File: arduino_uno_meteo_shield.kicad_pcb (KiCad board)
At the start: 2 copper layers, 14 parts

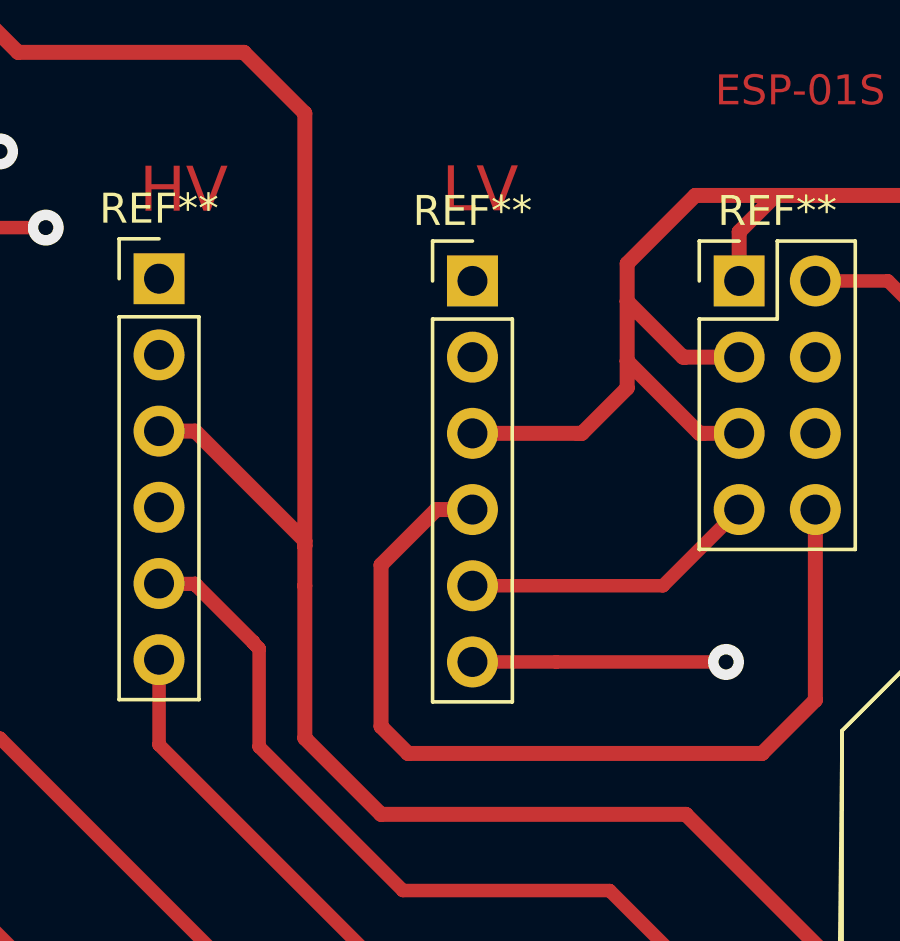
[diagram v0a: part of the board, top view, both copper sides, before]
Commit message: logic gate fix roaster
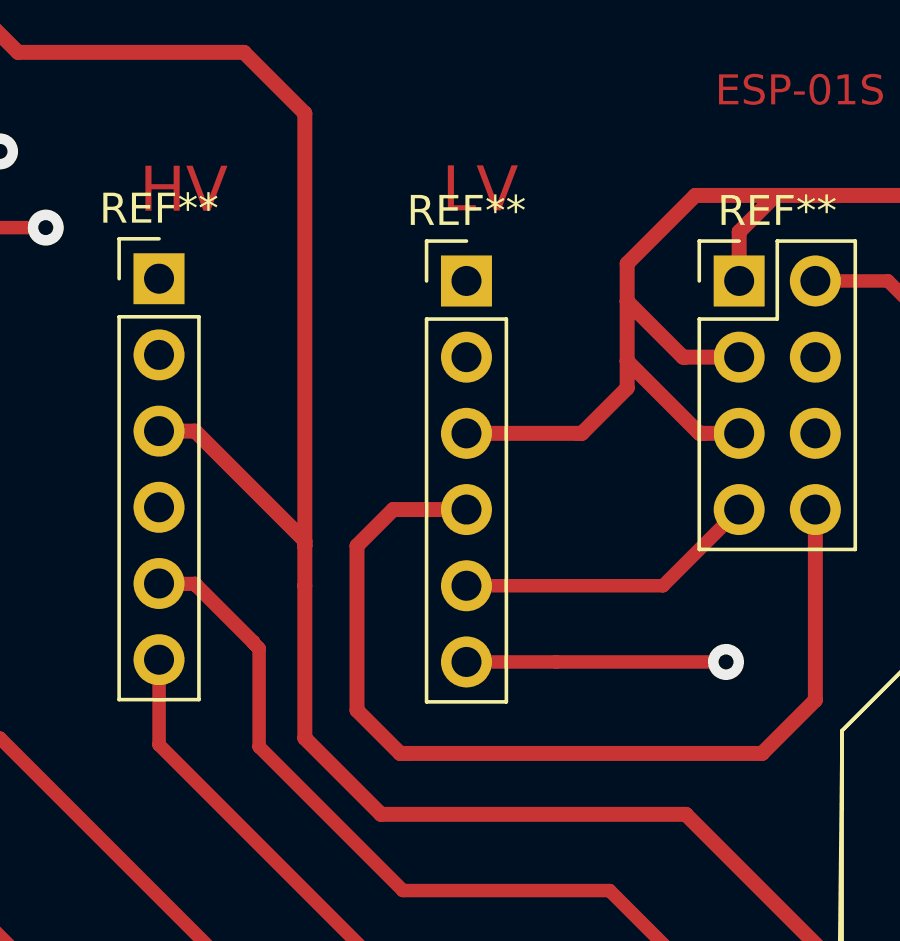
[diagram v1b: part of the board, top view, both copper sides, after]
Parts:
- moved REF** 0.20 mm to (167.9, 88.9)
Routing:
- net (no net): track 938.4 -> 939.9 mm
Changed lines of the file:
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@@
     (thickness 1.6)
     (drawings 21)
-    (tracks 251)
+    (tracks 252)
     (zones 0)
     (modules 14)
@@
   )
   (setup
-    (last_trace_width 0.45)
+    (last_trace_width 0.5)
     (user_trace_width 0.25)
     (user_trace_width 0.35)
@@
     (mod_text_width 0.15)
     (pad_size 1.7 1.7)
-    (pad_drill 1)
+    (pad_drill 0)
     (pad_to_mask_clearance 0.051)
     (solder_mask_min_width 0.25)
@@
     (pad 1 thru_hole rect (at 0 0) (size 1.7 1.7) (drill 1) (layers *.Cu *.Mask))
     (pad 2 thru_hole oval (at 0 2.54) (size 1.7 1.7) (drill 1) (layers *.Cu *.Mask))
-    (pad 3 thru_hole oval (at 0 5.08) (size 1.7 1.7) (drill 1) (layers *.Cu *.Mask))
+    (pad GND thru_hole oval (at 0 5.08) (size 1.7 1.7) (drill 1) (layers *.Cu *.Mask))
     (model ${KISYS3DMOD}/Connector_PinHeader_2.54mm.3dshapes/PinHeader_1x03_P2.54mm_Vertical.wrl
       (at (xyz 0 0 0))
@@
       (effects (font (size 1 1) (thickness 0.15)))
     )
-    (pad 1 thru_hole circle (at 0 0) (size 1.7 1.7) (drill 1) (layers *.Cu *.Mask))
+    (pad GND thru_hole circle (at 0 0) (size 1.7 1.7) (drill 1) (layers *.Cu *.Mask))
     (model ${KISYS3DMOD}/Connector_PinHeader_2.54mm.3dshapes/PinHeader_1x01_P2.54mm_Vertical.wrl
       (at (xyz 0 0 0))
@@
     (fp_line (start 1.27 -1.27) (end 1.27 39.37) (layer F.Fab) (width 0.1))
     (fp_line (start -0.635 -1.27) (end 1.27 -1.27) (layer F.Fab) (width 0.1))
-    (pad 16 thru_hole oval (at 0 38.1 90) (size 1.7 1.7) (drill 1) (layers *.Cu *.Mask))
+    (pad GND thru_hole oval (at 0 38.1 90) (size 1.7 1.7) (drill 1) (layers *.Cu *.Mask))
     (pad 15 thru_hole oval (at 0 35.56 90) (size 1.7 1.7) (drill 1) (layers *.Cu *.Mask))
     (pad 14 thru_hole oval (at 0 33.02 90) (size 1.7 1.7) (drill 1) (layers *.Cu *.Mask))
@@
     (pad 7 thru_hole oval (at 0 15.24 90) (size 1.7 1.7) (drill 1) (layers *.Cu *.Mask))
     (pad 6 thru_hole oval (at 0 12.7 90) (size 1.7 1.7) (drill 1) (layers *.Cu *.Mask))
-    (pad 5 thru_hole oval (at 0 10.16 90) (size 1.7 1.7) (drill 1) (layers *.Cu *.Mask))
+    (pad GND thru_hole oval (at 0 10.16 90) (size 1.7 1.7) (drill 1) (layers *.Cu *.Mask))
     (pad 4 thru_hole oval (at 0 7.62 90) (size 1.7 1.7) (drill 1) (layers *.Cu *.Mask))
     (pad 3 thru_hole oval (at 0 5.08 90) (size 1.7 1.7) (drill 1) (layers *.Cu *.Mask))
     (pad 2 thru_hole oval (at 0 2.54 90) (size 1.7 1.7) (drill 1) (layers *.Cu *.Mask))
-    (pad 1 thru_hole rect (at 0 0 90) (size 1.7 1.7) (drill 1) (layers *.Cu *.Mask))
+    (pad GND thru_hole rect (at 0 0 90) (size 1.7 1.7) (drill 1) (layers *.Cu *.Mask))
     (model ${KISYS3DMOD}/Connector_PinHeader_2.54mm.3dshapes/PinHeader_1x16_P2.54mm_Vertical.wrl
       (at (xyz 0 0 0))
@@
     (pad 6 thru_hole oval (at 0 12.7) (size 1.7 1.7) (drill 1) (layers *.Cu *.Mask))
     (pad 5 thru_hole oval (at 0 10.16) (size 1.7 1.7) (drill 1) (layers *.Cu *.Mask))
-    (pad 4 thru_hole oval (at 0 7.62) (size 1.7 1.7) (drill 1) (layers *.Cu *.Mask))
+    (pad GND thru_hole oval (at 0 7.62) (size 1.7 1.7) (drill 1) (layers *.Cu *.Mask))
     (pad 3 thru_hole oval (at 0 5.08) (size 1.7 1.7) (drill 1) (layers *.Cu *.Mask))
     (pad 2 thru_hole oval (at 0 2.54) (size 1.7 1.7) (drill 1) (layers *.Cu *.Mask))
@@
   )
   (module Connector_PinHeader_2.54mm:PinHeader_1x06_P2.54mm_Vertical (layer F.Cu)
-    (at 168.148 88.9)
+    (at 167.948 88.9)
     (descr "Through hole straight pin header, 1x06, 2.54mm pitch, single row")
     (tags "Through hole pin header THT 1x06 2.54mm single row")
@@
     (pad 3 thru_hole oval (at 0 5.08) (size 1.7 1.7) (drill 1) (layers *.Cu *.Mask))
     (pad 2 thru_hole oval (at 0 2.54) (size 1.7 1.7) (drill 1) (layers *.Cu *.Mask))
-    (pad 1 thru_hole rect (at 0 0) (size 1.7 1.7) (drill 1) (layers *.Cu *.Mask))
+    (pad GND thru_hole rect (at 0 0) (size 1.7 1.7) (drill 1) (layers *.Cu *.Mask))
     (model ${KISYS3DMOD}/Connector_PinHeader_2.54mm.3dshapes/PinHeader_1x03_P2.54mm_Vertical.wrl
       (at (xyz 0 0 0))
@@
     (pad 5 thru_hole oval (at 0 10.16) (size 1.7 1.7) (drill 1) (layers *.Cu *.Mask))
     (pad 4 thru_hole oval (at 0 7.62) (size 1.7 1.7) (drill 1) (layers *.Cu *.Mask))
-    (pad 3 thru_hole oval (at 0 5.08) (size 1.7 1.7) (drill 1) (layers *.Cu *.Mask))
+    (pad GND thru_hole oval (at 0 5.08) (size 1.7 1.7) (drill 1) (layers *.Cu *.Mask))
     (pad 2 thru_hole oval (at 0 2.54) (size 1.7 1.7) (drill 1) (layers *.Cu *.Mask))
     (pad 1 thru_hole rect (at 0 0) (size 1.7 1.7) (drill 1) (layers *.Cu *.Mask))
@@
     (pad 4 thru_hole oval (at 0 7.62) (size 1.7 1.7) (drill 1) (layers *.Cu *.Mask))
     (pad 3 thru_hole oval (at 0 5.08) (size 1.7 1.7) (drill 1) (layers *.Cu *.Mask))
-    (pad 2 thru_hole oval (at 0 2.54) (size 1.7 1.7) (drill 1) (layers *.Cu *.Mask))
+    (pad GND thru_hole oval (at 0 2.54) (size 1.7 1.7) (drill 1) (layers *.Cu *.Mask))
     (pad 1 thru_hole rect (at 0 0) (size 1.7 1.7) (drill 1) (layers *.Cu *.Mask))
     (model ${KISYS3DMOD}/Connector_PinHeader_2.54mm.3dshapes/PinHeader_1x04_P2.54mm_Vertical.wrl
@@
     (pad 4 thru_hole oval (at 0 7.62) (size 1.7 1.7) (drill 1) (layers *.Cu *.Mask))
     (pad 3 thru_hole oval (at 0 5.08) (size 1.7 1.7) (drill 1) (layers *.Cu *.Mask))
-    (pad 2 thru_hole oval (at 0 2.54) (size 1.7 1.7) (drill 1) (layers *.Cu *.Mask))
+    (pad GND thru_hole oval (at 0 2.54) (size 1.7 1.7) (drill 1) (layers *.Cu *.Mask))
     (pad 1 thru_hole rect (at 0 0) (size 1.7 1.7) (drill 1) (layers *.Cu *.Mask))
     (model ${KISYS3DMOD}/Connector_PinHeader_2.54mm.3dshapes/PinHeader_1x04_P2.54mm_Vertical.wrl
@@
   (segment (start 173.3042 91.5708) (end 173.3042 92.4708) (width 0.5) (layer F.Cu) (net 0))
   (segment (start 179.578 102.872) (end 179.578 96.52) (width 0.5) (layer F.Cu) (net 0))
-  (segment (start 166.945919 96.52) (end 165.1 98.365919) (width 0.5) (layer F.Cu) (net 0))
-  (segment (start 168.148 96.52) (end 166.945919 96.52) (width 0.5) (layer F.Cu) (net 0))
-  (segment (start 165.1 98.365919) (end 165.1 103.75) (width 0.5) (layer F.Cu) (net 0))
-  (segment (start 165.1 103.75) (end 166 104.65) (width 0.5) (layer F.Cu) (net 0))
   (segment (start 166 104.65) (end 177.8 104.65) (width 0.5) (layer F.Cu) (net 0))
   (segment (start 177.8 104.65) (end 179.578 102.872) (width 0.5) (layer F.Cu) (net 0))
@@
   (segment (start 132.588 101.6) (end 132.588 102.108) (width 0.45) (layer F.Cu) (net 0))
   (segment (start 132.588 101.6) (end 128.27 97.282) (width 0.45) (layer F.Cu) (net 0))
+  (segment (start 165.5064 96.52) (end 167.948 96.52) (width 0.5) (layer F.Cu) (net 0))
+  (segment (start 164.2999 97.7265) (end 165.5064 96.52) (width 0.5) (layer F.Cu) (net 0))
+  (segment (start 164.2999 103.2129) (end 164.2999 97.7265) (width 0.5) (layer F.Cu) (net 0))
+  (segment (start 166 104.65) (end 165.737 104.65) (width 0.5) (layer F.Cu) (net 0))
+  (segment (start 165.737 104.65) (end 164.2999 103.2129) (width 0.5) (layer F.Cu) (net 0))
   (zone (net 0) (net_name "") (layer F.Cu) (hatch edge 0.508)
     (connect_pads (clearance 0.508))

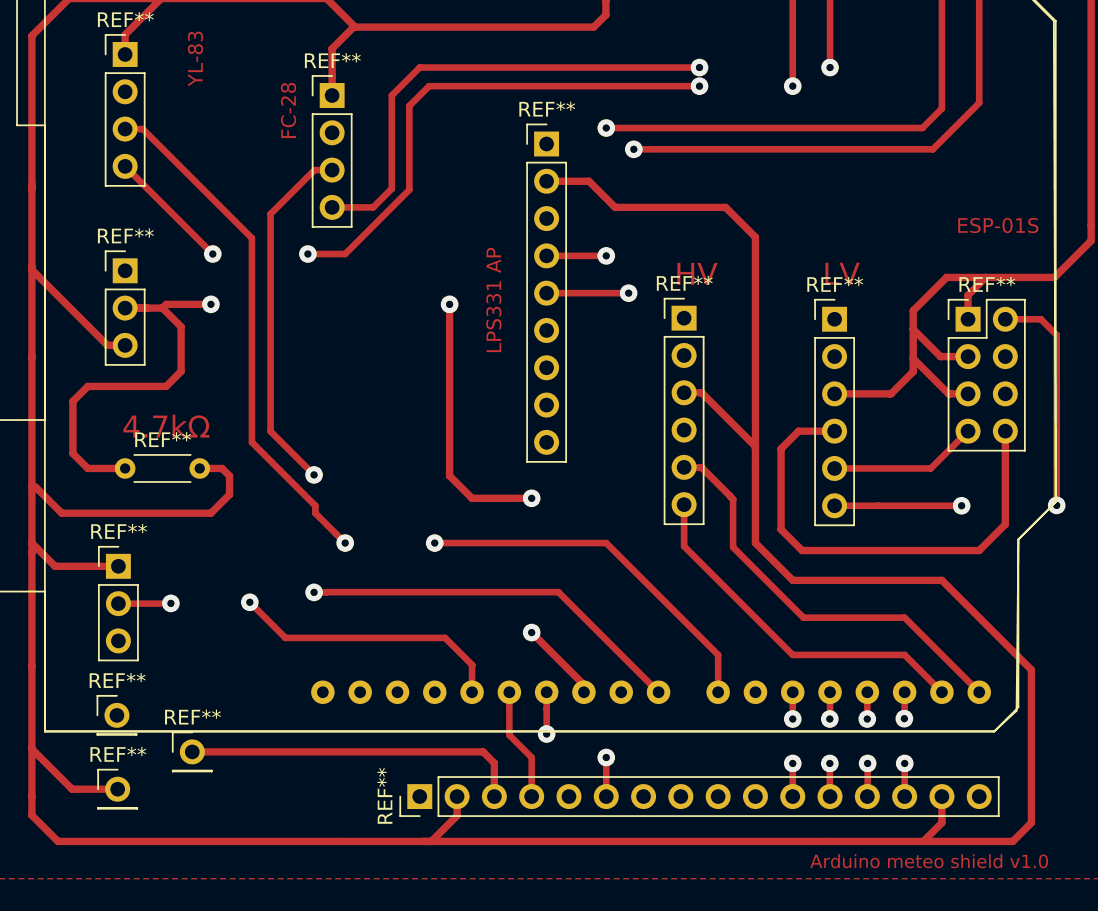
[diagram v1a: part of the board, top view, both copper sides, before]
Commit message: GND fix
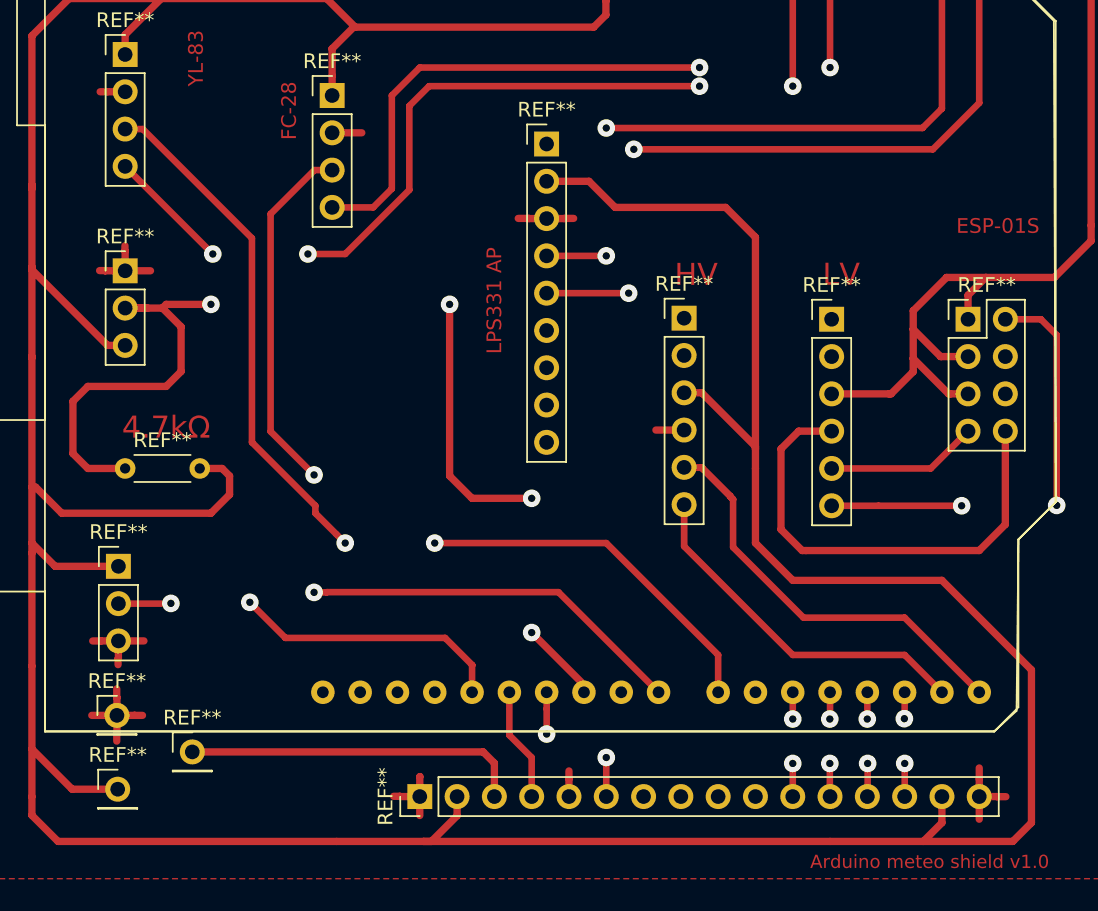
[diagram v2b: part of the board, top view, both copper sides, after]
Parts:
- moved REF** 0.20 mm to (167.7, 88.9)
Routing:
- net (no net): track 939.9 -> 978.1 mm
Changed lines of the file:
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@@
     (thickness 1.6)
     (drawings 21)
-    (tracks 252)
+    (tracks 300)
     (zones 0)
     (modules 14)
@@
   )
   (module Connector_PinHeader_2.54mm:PinHeader_1x06_P2.54mm_Vertical (layer F.Cu)
-    (at 167.948 88.9)
+    (at 167.748 88.9)
     (descr "Through hole straight pin header, 1x06, 2.54mm pitch, single row")
     (tags "Through hole pin header THT 1x06 2.54mm single row")
@@
   (segment (start 166 104.65) (end 165.737 104.65) (width 0.5) (layer F.Cu) (net 0))
   (segment (start 165.737 104.65) (end 164.2999 103.2129) (width 0.5) (layer F.Cu) (net 0))
+  (segment (start 119.634 73.406) (end 118.431919 73.406) (width 0.5) (layer F.Cu) (net 0))
+  (segment (start 118.431919 73.406) (end 117.9322 73.406) (width 0.5) (layer F.Cu) (net 0))
+  (segment (start 118.284 85.598) (end 118.2713 85.5853) (width 0.5) (layer F.Cu) (net 0))
+  (segment (start 119.634 85.598) (end 118.284 85.598) (width 0.5) (layer F.Cu) (net 0))
+  (segment (start 118.2713 85.5853) (end 117.8941 85.5853) (width 0.5) (layer F.Cu) (net 0))
+  (segment (start 119.634 85.598) (end 121.3612 85.598) (width 0.5) (layer F.Cu) (net 0))
+  (segment (start 119.634 84.248) (end 119.6213 84.2353) (width 0.5) (layer F.Cu) (net 0))
+  (segment (start 119.634 85.598) (end 119.634 84.248) (width 0.5) (layer F.Cu) (net 0))
+  (segment (start 119.6213 84.2353) (end 119.6213 83.8962) (width 0.5) (layer F.Cu) (net 0))
+  (segment (start 117.972919 110.805) (end 117.970419 110.8075) (width 0.5) (layer F.Cu) (net 0))
+  (segment (start 119.175 110.805) (end 117.972919 110.805) (width 0.5) (layer F.Cu) (net 0))
+  (segment (start 117.970419 110.8075) (end 117.4242 110.8075) (width 0.5) (layer F.Cu) (net 0))
+  (segment (start 119.175 110.805) (end 120.9142 110.805) (width 0.5) (layer F.Cu) (net 0))
+  (segment (start 119.175 112.007081) (end 119.1514 112.030681) (width 0.5) (layer F.Cu) (net 0))
+  (segment (start 119.175 110.805) (end 119.175 112.007081) (width 0.5) (layer F.Cu) (net 0))
+  (segment (start 119.1514 112.030681) (end 119.1514 112.4204) (width 0.5) (layer F.Cu) (net 0))
+  (segment (start 119.075 114.672919) (end 119.0625 114.660419) (width 0.5) (layer F.Cu) (net 0))
+  (segment (start 119.075 115.875) (end 119.075 114.672919) (width 0.5) (layer F.Cu) (net 0))
+  (segment (start 119.0625 114.660419) (end 119.0625 114.0714) (width 0.5) (layer F.Cu) (net 0))
+  (segment (start 119.075 117.077081) (end 119.0625 117.089581) (width 0.5) (layer F.Cu) (net 0))
+  (segment (start 119.075 115.875) (end 119.075 117.077081) (width 0.5) (layer F.Cu) (net 0))
+  (segment (start 119.0625 117.089581) (end 119.0625 117.6274) (width 0.5) (layer F.Cu) (net 0))
+  (segment (start 119.075 115.875) (end 117.3609 115.875) (width 0.5) (layer F.Cu) (net 0))
+  (segment (start 120.277081 115.875) (end 120.277281 115.8748) (width 0.5) (layer F.Cu) (net 0))
+  (segment (start 119.075 115.875) (end 120.277081 115.875) (width 0.5) (layer F.Cu) (net 0))
+  (segment (start 120.277281 115.8748) (end 120.8151 115.8748) (width 0.5) (layer F.Cu) (net 0))
+  (segment (start 138.35 121.404) (end 138.3326 121.3866) (width 0.5) (layer F.Cu) (net 0))
+  (segment (start 139.7 121.404) (end 138.35 121.404) (width 0.5) (layer F.Cu) (net 0))
+  (segment (start 138.3326 121.3866) (end 137.922 121.3866) (width 0.5) (layer F.Cu) (net 0))
+  (segment (start 149.86 121.404) (end 149.86 120.201919) (width 0.5) (layer F.Cu) (net 0))
+  (segment (start 149.86 120.201919) (end 149.86 119.6594) (width 0.5) (layer F.Cu) (net 0))
+  (segment (start 177.8 121.404) (end 177.8 120.201919) (width 0.5) (layer F.Cu) (net 0))
+  (segment (start 177.8 120.201919) (end 177.8 119.4562) (width 0.5) (layer F.Cu) (net 0))
+  (segment (start 179.002081 121.404) (end 179.010081 121.412) (width 0.5) (layer F.Cu) (net 0))
+  (segment (start 177.8 121.404) (end 179.002081 121.404) (width 0.5) (layer F.Cu) (net 0))
+  (segment (start 179.010081 121.412) (end 179.6161 121.412) (width 0.5) (layer F.Cu) (net 0))
+  (segment (start 133.731 76.2) (end 135.7503 76.2) (width 0.5) (layer F.Cu) (net 0))
+  (segment (start 147.133919 82.042) (end 147.121219 82.0293) (width 0.5) (layer F.Cu) (net 0))
+  (segment (start 148.336 82.042) (end 147.133919 82.042) (width 0.5) (layer F.Cu) (net 0))
+  (segment (start 147.121219 82.0293) (end 146.4056 82.0293) (width 0.5) (layer F.Cu) (net 0))
+  (segment (start 149.538081 82.042) (end 149.550781 82.0293) (width 0.5) (layer F.Cu) (net 0))
+  (segment (start 148.336 82.042) (end 149.538081 82.042) (width 0.5) (layer F.Cu) (net 0))
+  (segment (start 149.550781 82.0293) (end 150.1775 82.0293) (width 0.5) (layer F.Cu) (net 0))
+  (segment (start 157.7 96.445) (end 155.7794 96.445) (width 0.5) (layer F.Cu) (net 0))
+  (segment (start 177.8 121.404) (end 177.8 122.9487) (width 0.5) (layer F.Cu) (net 0))
+  (segment (start 139.7 120.054) (end 139.7127 120.0413) (width 0.5) (layer F.Cu) (net 0))
+  (segment (start 139.7 121.404) (end 139.7 120.054) (width 0.5) (layer F.Cu) (net 0))
+  (segment (start 139.7 121.404) (end 139.7 122.6947) (width 0.5) (layer F.Cu) (net 0))
   (zone (net 0) (net_name "") (layer F.Cu) (hatch edge 0.508)
     (connect_pads (clearance 0.508))
